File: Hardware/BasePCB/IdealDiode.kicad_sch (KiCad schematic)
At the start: 9 parts, among them IC1 AP74502HQTA8-7, Q5 SQJQ140E-T1_GE3, Q6 SQJQ140E-T1_GE3

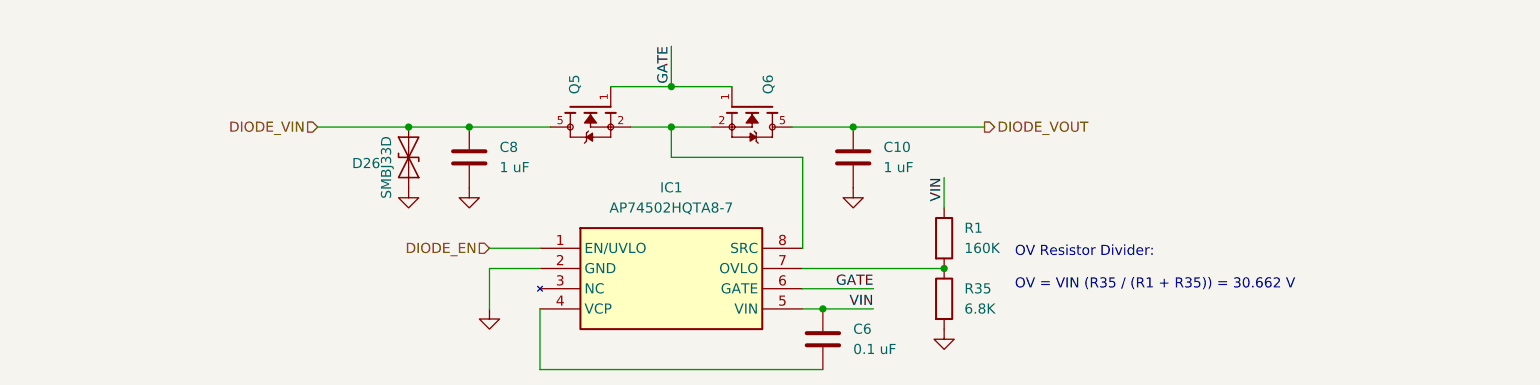
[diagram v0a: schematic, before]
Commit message: donut daddy
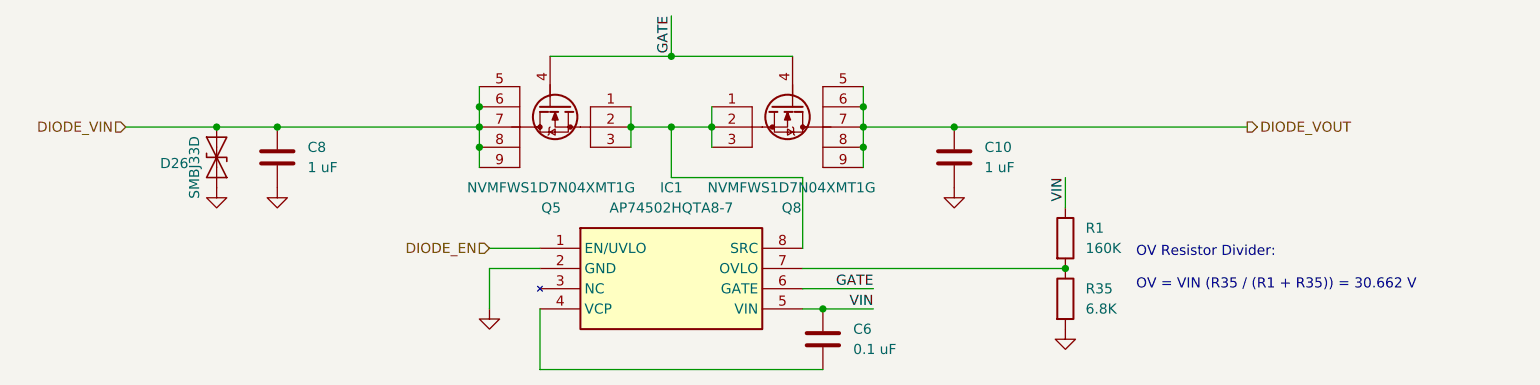
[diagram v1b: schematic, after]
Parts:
- removed Q5, Q6: SQJQ140E-T1_GE3, PowerBoardLib:TO200P800X182-5N, symbol PowerBoardLib:SQJQ140E-T1_GE3
- added Q5, Q8: NVMFWS1D7N04XMT1G, LV Carrier Library:NVMFWS3D0P04M8LT1G, symbol NVMFWS1D7N04XMT1G:NVMFWS1D7N04XMT1G
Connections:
- net DIODE_VIN: now also Q5.5, Q5.6, Q5.7, Q5.8, Q5.9
- net DIODE_VOUT: now also Q8.5, Q8.6, Q8.7, Q8.8, Q8.9
- net GATE: now also Q5.4, Q8.4
- net at IC1.8 (SRC): now also Q5.1, Q5.2, Q5.3, Q8.1, Q8.2, Q8.3
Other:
- moved on the sheet: C10, C8, D26, R1, R35
